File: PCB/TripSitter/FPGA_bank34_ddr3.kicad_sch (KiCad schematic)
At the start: 12 parts, among them IC2 MT41J128M16JT-125_K, U1 XC7A100T-FGG484, X1 XO53 100Mhz

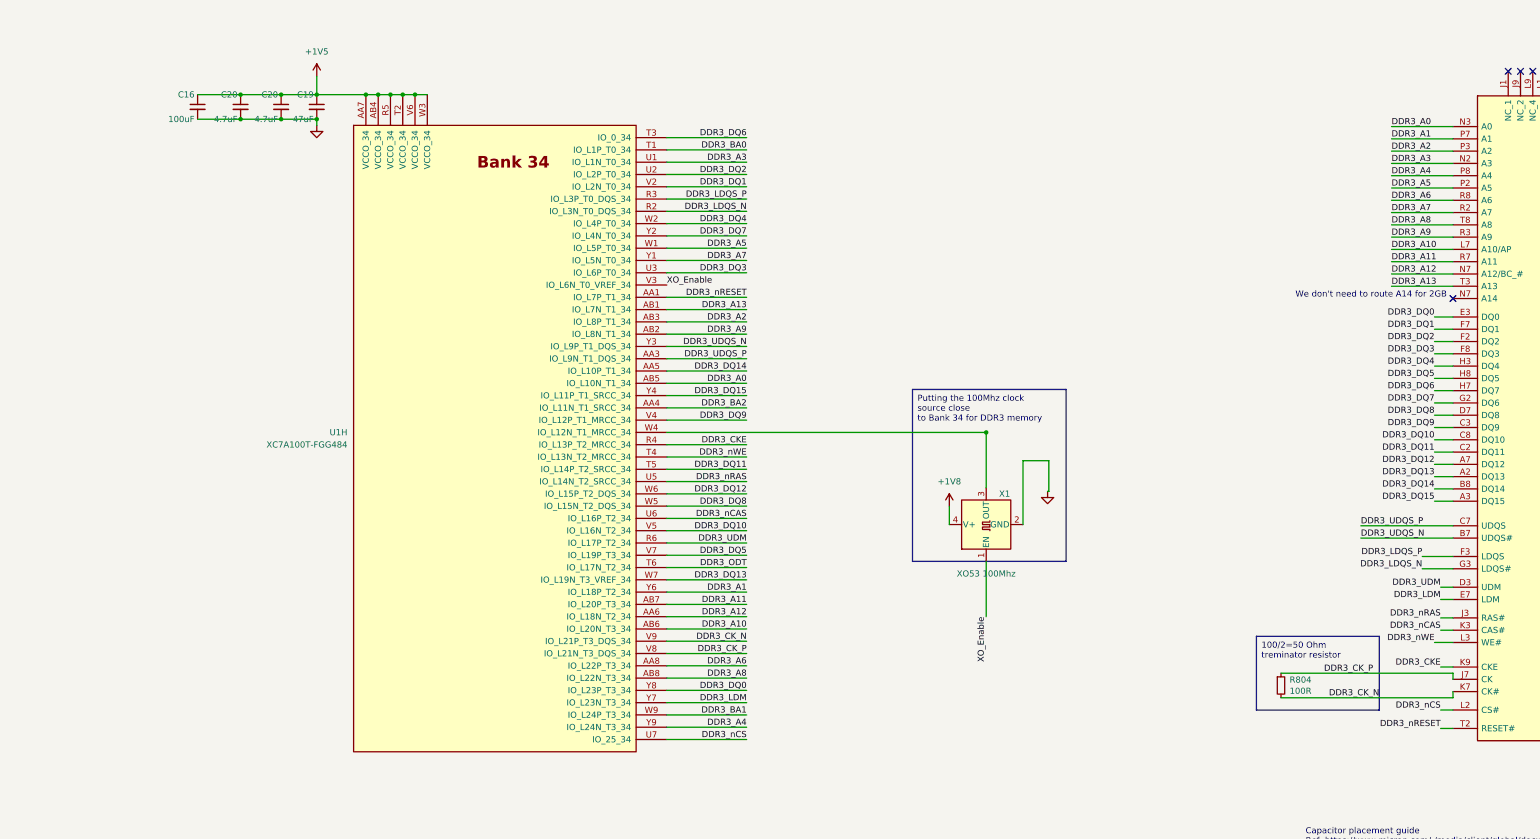
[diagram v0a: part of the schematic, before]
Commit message: more pcb routing
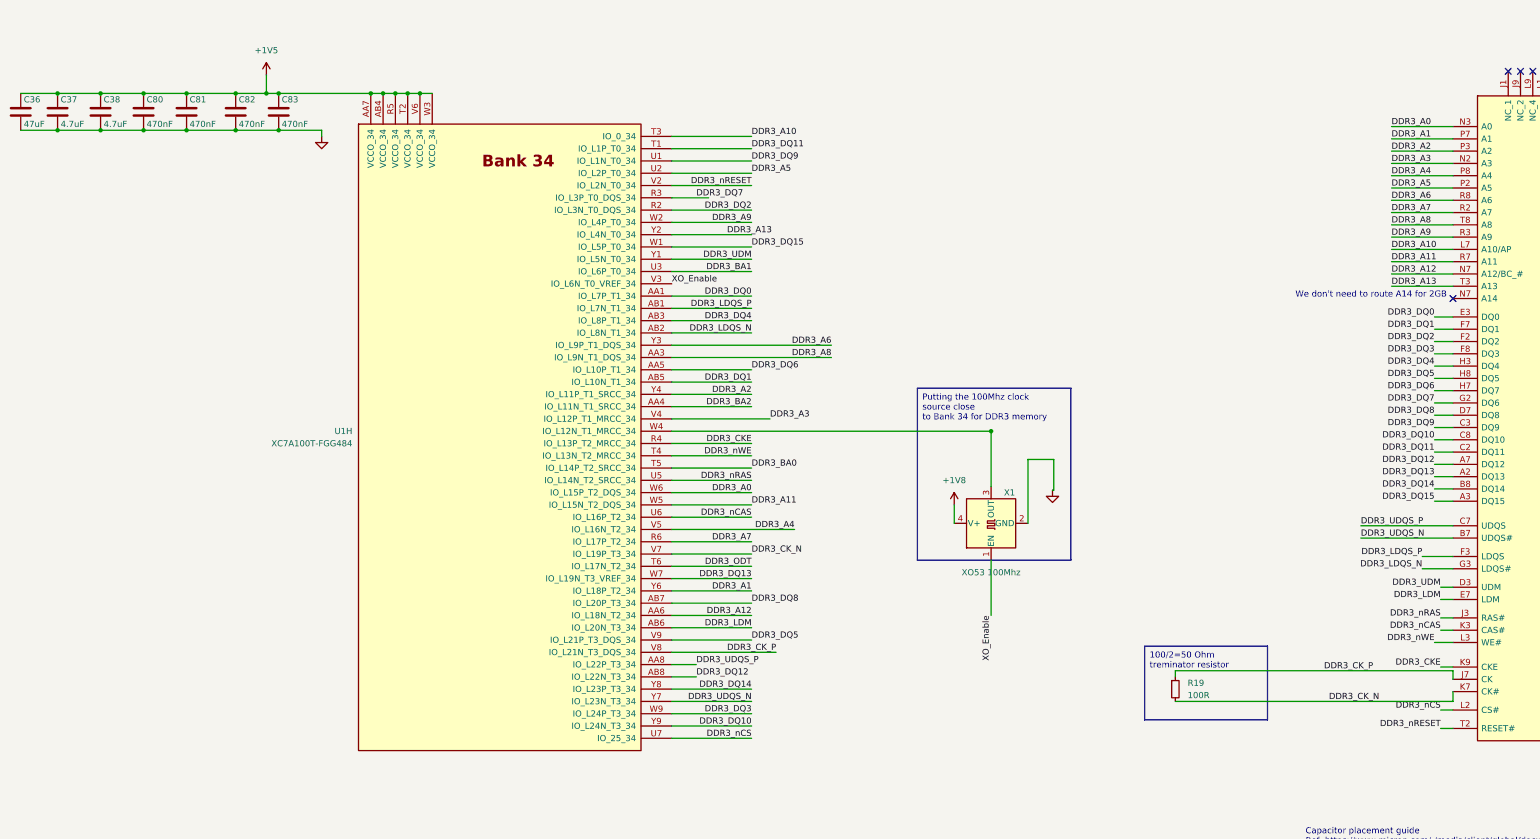
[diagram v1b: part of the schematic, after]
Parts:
- removed C16: 100uF, Capacitor_SMD:C_1210_3225Metric_Pad1.33x2.70mm_HandSolder, symbol Device:C_Small
- removed C19: 47uF, Capacitor_SMD:C_1210_3225Metric_Pad1.33x2.70mm_HandSolder, symbol Device:C_Small
- removed C20 (x2): 4.7uF, Capacitor_SMD:C_0805_2012Metric_Pad1.18x1.45mm_HandSolder, symbol Device:C_Small
- removed R804: 100R, Resistor_SMD:R_0201_0603Metric_Pad0.64x0.40mm_HandSolder, symbol Device:R_Small
- added C36: 47uF, Capacitor_SMD:C_1210_3225Metric_Pad1.33x2.70mm_HandSolder, symbol Device:C
- added C37, C38: 4.7uF, Capacitor_SMD:C_0805_2012Metric_Pad1.18x1.45mm_HandSolder, symbol Device:C
- added C80, C81, C82, C83: 470nF, Capacitor_SMD:C_0201_0603Metric_Pad0.64x0.40mm_HandSolder, symbol Device:C
- added R19: 100R, symbol Device:R_Small
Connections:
- net +1V5: now also C36.1, C37.1, C38.1, C80.1, C81.1, C82.1, C83.1
- net DDR3_A0: now also U1.W6 (IO_L15P_T2_DQS_34); no longer U1.AB5 (IO_L10N_T1_34)
- net DDR3_A10: now also U1.T3 (IO_0_34); no longer U1.AB6 (IO_L20N_T3_34)
- net DDR3_A11: now also U1.W5 (IO_L15N_T2_DQS_34); no longer U1.AB7 (IO_L20P_T3_34)
- net DDR3_A13: now also U1.Y2 (IO_L4N_T0_34); no longer U1.AB1 (IO_L7N_T1_34)
- net DDR3_A2: now also U1.Y4 (IO_L11P_T1_SRCC_34); no longer U1.AB3 (IO_L8P_T1_34)
- net DDR3_A3: now also U1.V4 (IO_L12P_T1_MRCC_34); no longer U1.U1 (IO_L1N_T0_34)
- net DDR3_A4: now also U1.V5 (IO_L16N_T2_34); no longer U1.Y9 (IO_L24N_T3_34)
- net DDR3_A5: now also U1.U2 (IO_L2P_T0_34); no longer U1.W1 (IO_L5P_T0_34)
- net DDR3_A6: now also U1.Y3 (IO_L9P_T1_DQS_34); no longer U1.AA8 (IO_L22P_T3_34)
- net DDR3_A7: now also U1.R6 (IO_L17P_T2_34); no longer U1.Y1 (IO_L5N_T0_34)
- net DDR3_A8: now also U1.AA3 (IO_L9N_T1_DQS_34); no longer U1.AB8 (IO_L22N_T3_34)
- net DDR3_A9: now also U1.W2 (IO_L4P_T0_34); no longer U1.AB2 (IO_L8N_T1_34)
- net DDR3_BA0: now also U1.T5 (IO_L14P_T2_SRCC_34); no longer U1.T1 (IO_L1P_T0_34)
- net DDR3_BA1: now also U1.U3 (IO_L6P_T0_34); no longer U1.W9 (IO_L24P_T3_34)
- net DDR3_CK_N: now also U1.V7 (IO_L19P_T3_34), R19.2; no longer U1.V9 (IO_L21P_T3_DQS_34)
- net DDR3_CK_P: now also R19.1
- net DDR3_DQ0: now also U1.AA1 (IO_L7P_T1_34); no longer U1.Y8 (IO_L23P_T3_34)
- net DDR3_DQ1: now also U1.AB5 (IO_L10N_T1_34); no longer U1.V2 (IO_L2N_T0_34)
- net DDR3_DQ10: now also U1.Y9 (IO_L24N_T3_34); no longer U1.V5 (IO_L16N_T2_34)
- net DDR3_DQ11: now also U1.T1 (IO_L1P_T0_34); no longer U1.T5 (IO_L14P_T2_SRCC_34)
- net DDR3_DQ12: now also U1.AB8 (IO_L22N_T3_34); no longer U1.W6 (IO_L15P_T2_DQS_34)
- net DDR3_DQ14: now also U1.Y8 (IO_L23P_T3_34); no longer U1.AA5 (IO_L10P_T1_34)
- net DDR3_DQ15: now also U1.W1 (IO_L5P_T0_34); no longer U1.Y4 (IO_L11P_T1_SRCC_34)
- net DDR3_DQ2: now also U1.R2 (IO_L3N_T0_DQS_34); no longer U1.U2 (IO_L2P_T0_34)
- net DDR3_DQ3: now also U1.W9 (IO_L24P_T3_34); no longer U1.U3 (IO_L6P_T0_34)
- net DDR3_DQ4: now also U1.AB3 (IO_L8P_T1_34); no longer U1.W2 (IO_L4P_T0_34)
- net DDR3_DQ5: now also U1.V9 (IO_L21P_T3_DQS_34); no longer U1.V7 (IO_L19P_T3_34)
- net DDR3_DQ6: now also U1.AA5 (IO_L10P_T1_34); no longer U1.T3 (IO_0_34)
- net DDR3_DQ7: now also U1.R3 (IO_L3P_T0_DQS_34); no longer U1.Y2 (IO_L4N_T0_34)
- net DDR3_DQ8: now also U1.AB7 (IO_L20P_T3_34); no longer U1.W5 (IO_L15N_T2_DQS_34)
- net DDR3_DQ9: now also U1.U1 (IO_L1N_T0_34); no longer U1.V4 (IO_L12P_T1_MRCC_34)
- net DDR3_LDM: now also U1.AB6 (IO_L20N_T3_34); no longer U1.Y7 (IO_L23N_T3_34)
- net DDR3_LDQS_N: now also U1.AB2 (IO_L8N_T1_34); no longer U1.R2 (IO_L3N_T0_DQS_34)
- net DDR3_LDQS_P: now also U1.AB1 (IO_L7N_T1_34); no longer U1.R3 (IO_L3P_T0_DQS_34)
- net DDR3_UDM: now also U1.Y1 (IO_L5N_T0_34); no longer U1.R6 (IO_L17P_T2_34)
- net DDR3_UDQS_N: now also U1.Y7 (IO_L23N_T3_34); no longer U1.Y3 (IO_L9P_T1_DQS_34)
- net DDR3_UDQS_P: now also U1.AA8 (IO_L22P_T3_34); no longer U1.AA3 (IO_L9N_T1_DQS_34)
- net DDR3_nRESET: now also U1.V2 (IO_L2N_T0_34); no longer U1.AA1 (IO_L7P_T1_34)
- net GND: now also C36.2, C37.2, C38.2, C80.2, C81.2, C82.2, C83.2
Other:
- moved on the sheet: U1H, X1
